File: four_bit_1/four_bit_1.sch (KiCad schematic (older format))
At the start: 1 part, among them P1 DIN_41612_128P

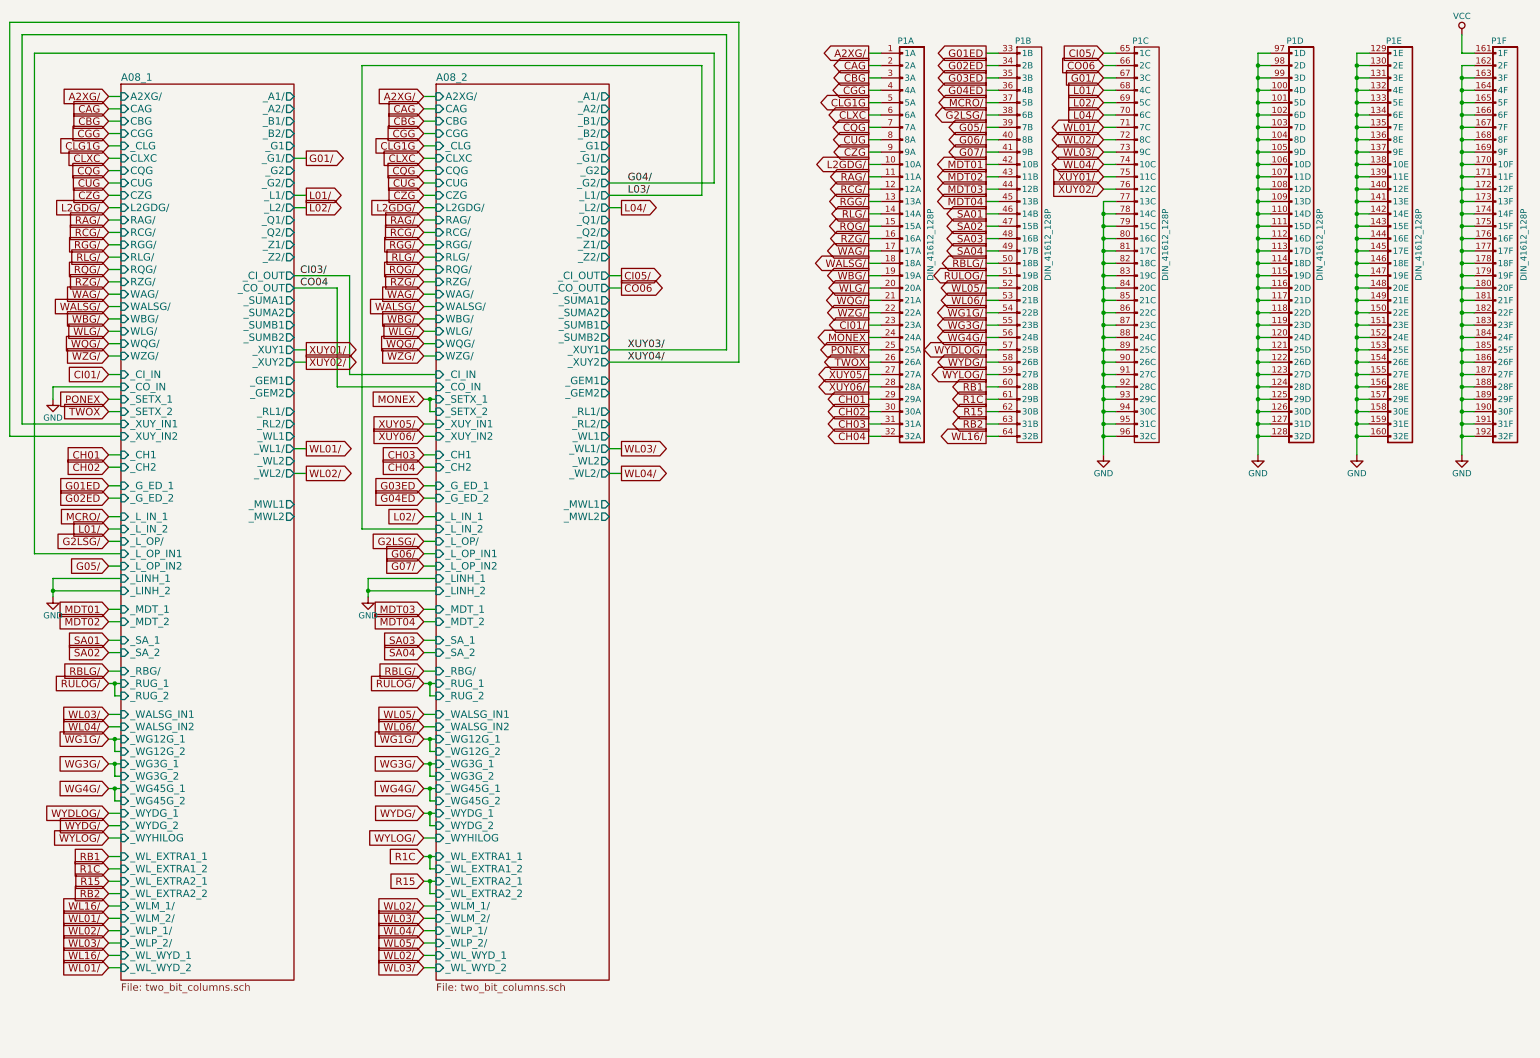
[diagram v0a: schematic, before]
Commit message: Added in WHOMP, whatever it is
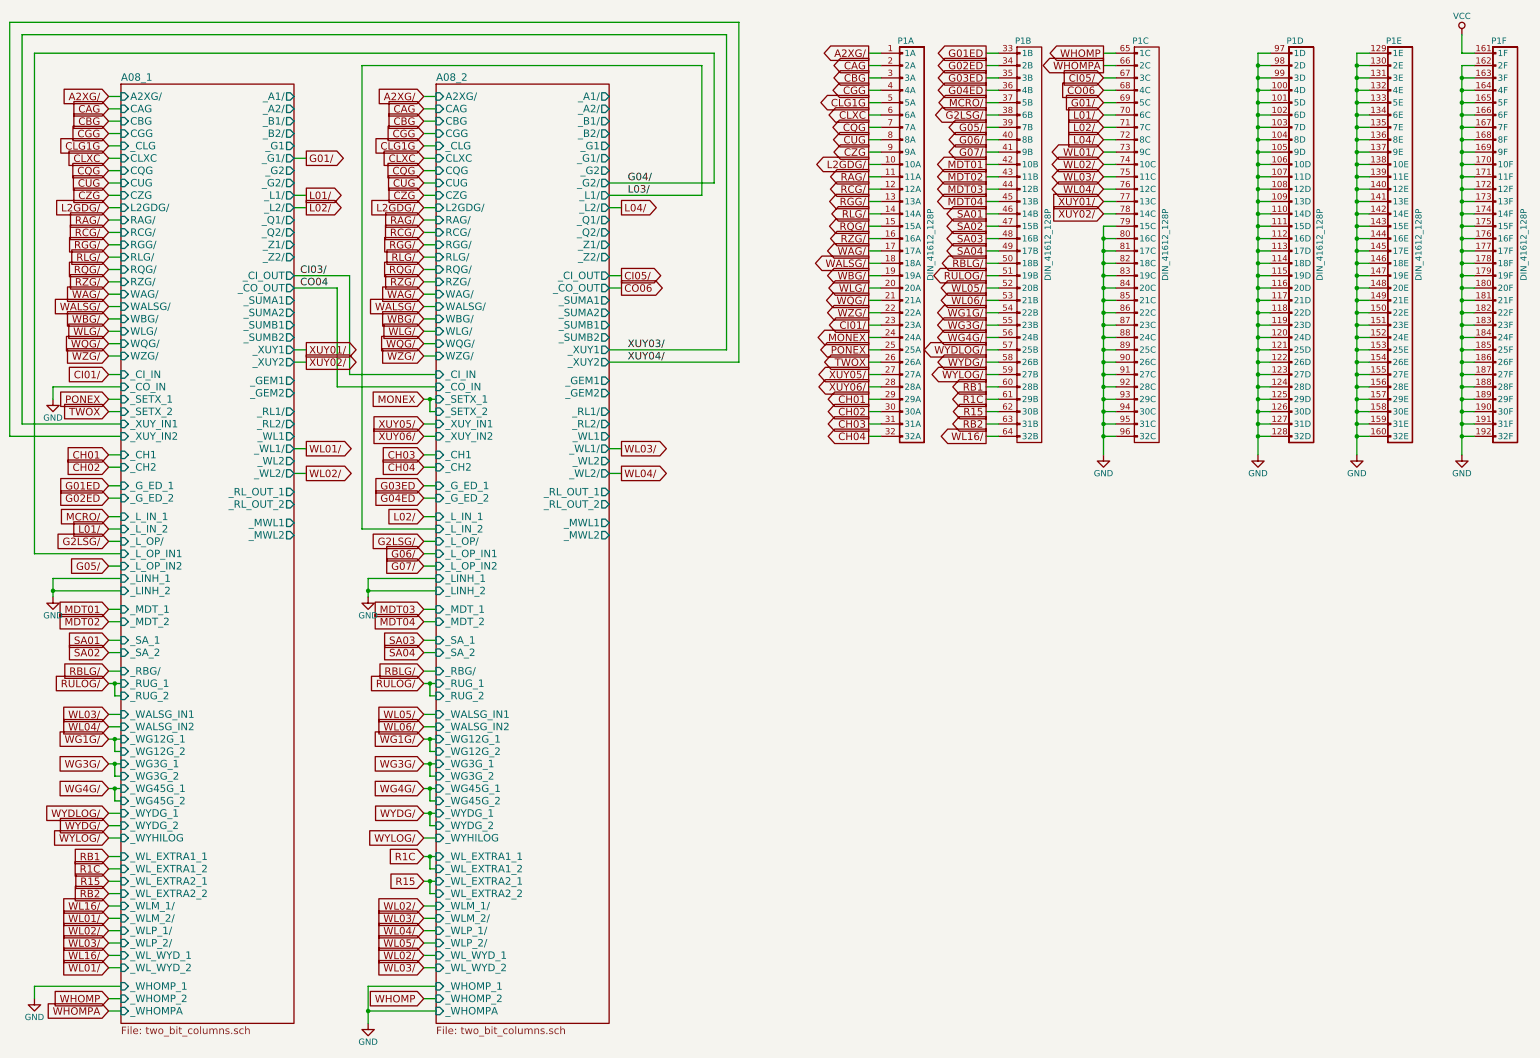
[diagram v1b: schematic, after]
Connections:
- net CI05/: now also P1.67 (3C); no longer P1.65 (1C)
- net CO06: now also P1.68 (4C); no longer P1.66 (2C)
- net G01/: now also P1.69 (5C); no longer P1.67 (3C)
- net GND: no longer P1.77 (13C), P1.78 (14C)
- net L01/: now also P1.70 (6C); no longer P1.68 (4C)
- net L02/: now also P1.71 (7C); no longer P1.69 (5C)
- net L04/: now also P1.72 (8C); no longer P1.70 (6C)
- net WL01/: now also P1.73 (9C); no longer P1.71 (7C)
- net WL02/: now also P1.74 (10C); no longer P1.72 (8C)
- net WL03/: now also P1.75 (11C); no longer P1.73 (9C)
- net WL04/: now also P1.76 (12C); no longer P1.74 (10C)
- net XUY01/: now also P1.77 (13C); no longer P1.75 (11C)
- net XUY02/: now also P1.78 (14C); no longer P1.76 (12C)
- new net WHOMP: P1.65 (1C)
- new net WHOMPA: P1.66 (2C)
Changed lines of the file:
@@
 $EndDescr
 $Sheet
-S 1750 1200 1400 7250
+S 1750 1200 1400 7600
 U 5684C508
 F0 "A08_1" 60
@@
 F60 "_WL1" O R 3150 4050 60
 F61 "_WL1/" O R 3150 4150 60
-F62 "_MWL1" O R 3150 4600 60
+F62 "_MWL1" O R 3150 4750 60
 F63 "_CI_OUT" O R 3150 2750 60
 F64 "_CO_IN" I L 1750 3650 60
@@
 F96 "_WL2" O R 3150 4250 60
 F97 "_WL2/" O R 3150 4350 60
-F98 "_MWL2" O R 3150 4700 60
+F98 "_MWL2" O R 3150 4850 60
 F99 "_RL1/" O R 3150 3850 60
 F100 "_RL2/" O R 3150 3950 60
+F101 "_RL_OUT_2" O R 3150 4600 60
+F102 "_RL_OUT_1" O R 3150 4500 60
+F103 "_WHOMPA" I L 1750 8700 60
+F104 "_WHOMP_1" I L 1750 8500 60
+F105 "_WHOMP_2" I L 1750 8600 60
 $EndSheet
 $Comp
@@
 $EndComp
 $Sheet
-S 4300 1200 1400 7250
+S 4300 1200 1400 7600
 U 5689EF80
 F0 "A08_2" 60
@@
 F60 "_WL1" O R 5700 4050 60
 F61 "_WL1/" O R 5700 4150 60
-F62 "_MWL1" O R 5700 4600 60
+F62 "_MWL1" O R 5700 4750 60
 F63 "_CI_OUT" O R 5700 2750 60
 F64 "_CO_IN" I L 4300 3650 60
@@
 F96 "_WL2" O R 5700 4250 60
 F97 "_WL2/" O R 5700 4350 60
-F98 "_MWL2" O R 5700 4700 60
+F98 "_MWL2" O R 5700 4850 60
 F99 "_RL1/" O R 5700 3850 60
 F100 "_RL2/" O R 5700 3950 60
+F101 "_RL_OUT_2" O R 5700 4600 60
+F102 "_RL_OUT_1" O R 5700 4500 60
+F103 "_WHOMPA" I L 4300 8700 60
+F104 "_WHOMP_1" I L 4300 8500 60
+F105 "_WHOMP_2" I L 4300 8600 60
 $EndSheet
 Text GLabel 1650 1300 0    60   Input ~ 0
@@
 $EndComp
 Wire Wire Line
-	9700 2150 9800 2150
-Wire Wire Line
-	9700 2250 9800 2250
-Connection ~ 9700 2250
-Wire Wire Line
 	9700 2350 9800 2350
-Connection ~ 9700 2350
 Wire Wire Line
 	9700 2450 9800 2450
@@
 Text Label 5850 2000 0    60   ~ 0
 G04/
-Text GLabel 9700 1250 0    60   Input ~ 0
+Text GLabel 9700 1450 0    60   Input ~ 0
 L01/
 Wire Wire Line
-	9800 1250 9700 1250
-Text GLabel 9700 1350 0    60   Input ~ 0
+	9800 1450 9700 1450
+Text GLabel 9700 1550 0    60   Input ~ 0
 L02/
 Wire Wire Line
-	9800 1350 9700 1350
-Wire Wire Line
-	9700 2150 9700 4200
-Text GLabel 9700 1550 0    60   BiDi ~ 0
+	9800 1550 9700 1550
+Wire Wire Line
+	9700 2350 9700 4200
+Text GLabel 9700 1750 0    60   BiDi ~ 0
 WL01/
-Wire Wire Line
-	9800 1550 9700 1550
-Text GLabel 9700 1650 0    60   BiDi ~ 0
-WL02/
-Wire Wire Line
-	9800 1650 9700 1650
-Text GLabel 9700 1750 0    60   BiDi ~ 0
-WL03/
 Wire Wire Line
 	9800 1750 9700 1750
 Text GLabel 9700 1850 0    60   BiDi ~ 0
+WL02/
+Wire Wire Line
+	9800 1850 9700 1850
+Text GLabel 9700 1950 0    60   BiDi ~ 0
+WL03/
+Wire Wire Line
+	9800 1950 9700 1950
+Text GLabel 9700 2050 0    60   BiDi ~ 0
 WL04/
 Wire Wire Line
-	9800 1850 9700 1850
+	9800 2050 9700 2050
 Text GLabel 5800 2750 2    60   Output ~ 0
 CI05/
@@
 Wire Wire Line
 	5700 2850 5800 2850
-Text GLabel 9700 950  0    60   Input ~ 0
+Text GLabel 9700 1150 0    60   Input ~ 0
 CI05/
 Wire Wire Line
-	9800 950  9700 950
-Text GLabel 9700 1050 0    60   Input ~ 0
+	9800 1150 9700 1150
+Text GLabel 9700 1250 0    60   Input ~ 0
 CO06
 Wire Wire Line
-	9800 1050 9700 1050
+	9800 1250 9700 1250
 Text GLabel 5800 2200 2    60   Output ~ 0
 L04/
 Wire Wire Line
 	5700 2200 5800 2200
-Text GLabel 9700 1450 0    60   Input ~ 0
+Text GLabel 9700 1650 0    60   Input ~ 0
 L04/
 Wire Wire Line
-	9800 1450 9700 1450
+	9800 1650 9700 1650
 Wire Wire Line
 	3150 1800 3250 1800
 Text GLabel 3250 1800 2    60   Output ~ 0
 G01/
-Text GLabel 9700 1150 0    60   Input ~ 0
+Text GLabel 9700 1350 0    60   Input ~ 0
 G01/
 Wire Wire Line
-	9800 1150 9700 1150
+	9800 1350 9700 1350
 Text GLabel 3250 3350 2    60   Output ~ 0
 XUY01/
@@
 Wire Wire Line
 	3150 3450 3250 3450
-Text GLabel 9700 1950 0    60   Input ~ 0
+Text GLabel 9700 2150 0    60   Input ~ 0
 XUY01/
 Wire Wire Line
-	9800 1950 9700 1950
-Text GLabel 9700 2050 0    60   Input ~ 0
+	9800 2150 9700 2150
+Text GLabel 9700 2250 0    60   Input ~ 0
 XUY02/
 Wire Wire Line
-	9800 2050 9700 2050
+	9800 2250 9700 2250
+Text GLabel 1650 8700 0    60   Input ~ 0
+WHOMPA
+Wire Wire Line
+	1750 8700 1650 8700
+$Comp
+L GND #PWR09
+U 1 1 56BB3258
+P 3750 8800
+F 0 "#PWR09" H 3750 8550 50  0001 C CNN
+F 1 "GND" H 3750 8650 50  0000 C CNN
+F 2 "" H 3750 8800 60  0000 C CNN
+F 3 "" H 3750 8800 60  0000 C CNN
+	1    3750 8800
+	1    0    0    -1
+$EndComp
+Wire Wire Line
+	4300 8700 3750 8700
+Text GLabel 1650 8600 0    60   Input ~ 0
+WHOMP
+Wire Wire Line
+	1750 8600 1650 8600
+$Comp
+L GND #PWR010
+U 1 1 56C05747
+P 1050 8600
+F 0 "#PWR010" H 1050 8350 50  0001 C CNN
+F 1 "GND" H 1050 8450 50  0000 C CNN
+F 2 "" H 1050 8600 60  0000 C CNN
+F 3 "" H 1050 8600 60  0000 C CNN
+	1    1050 8600
+	1    0    0    -1
+$EndComp
+Wire Wire Line
+	1750 8500 1050 8500
+Wire Wire Line
+	1050 8500 1050 8600
+Connection ~ 3750 8700
+Text GLabel 4200 8600 0    60   Input ~ 0
+WHOMP
+Wire Wire Line
+	4300 8600 4200 8600
+Wire Wire Line
+	3750 8500 3750 8800
+Wire Wire Line
+	3750 8500 4300 8500
+Text GLabel 9700 950  0    60   Output ~ 0
+WHOMP
+Wire Wire Line
+	9800 950  9700 950
+Text GLabel 9700 1050 0    60   Output ~ 0
+WHOMPA
+Wire Wire Line
+	9800 1050 9700 1050
 $EndSCHEMATC
